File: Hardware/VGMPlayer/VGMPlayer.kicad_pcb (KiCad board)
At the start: 2 copper layers, 110.7 x 70.6 mm, 92 parts, among them J1 USB_B_Mini, J2 SD_Card, Q1 9013, Q2 S8550, SW1 Mode, SW2 NEXT, SW3 PREV, SW4 SELECT, SW5 PWR, U1 STM32F103XX, U10 LTC6903, U11 HC-06, U13 YM3012, U14 LM324, U18 OLED_128_64_I2C, U19 ESP8266Module, U2 SDCardModule, U3 LM386, U4 LM386, U5 YM2151, U6 AUDIOJACK-VGM, U7 YM2612, U8 SN76489, U9 LTC6903

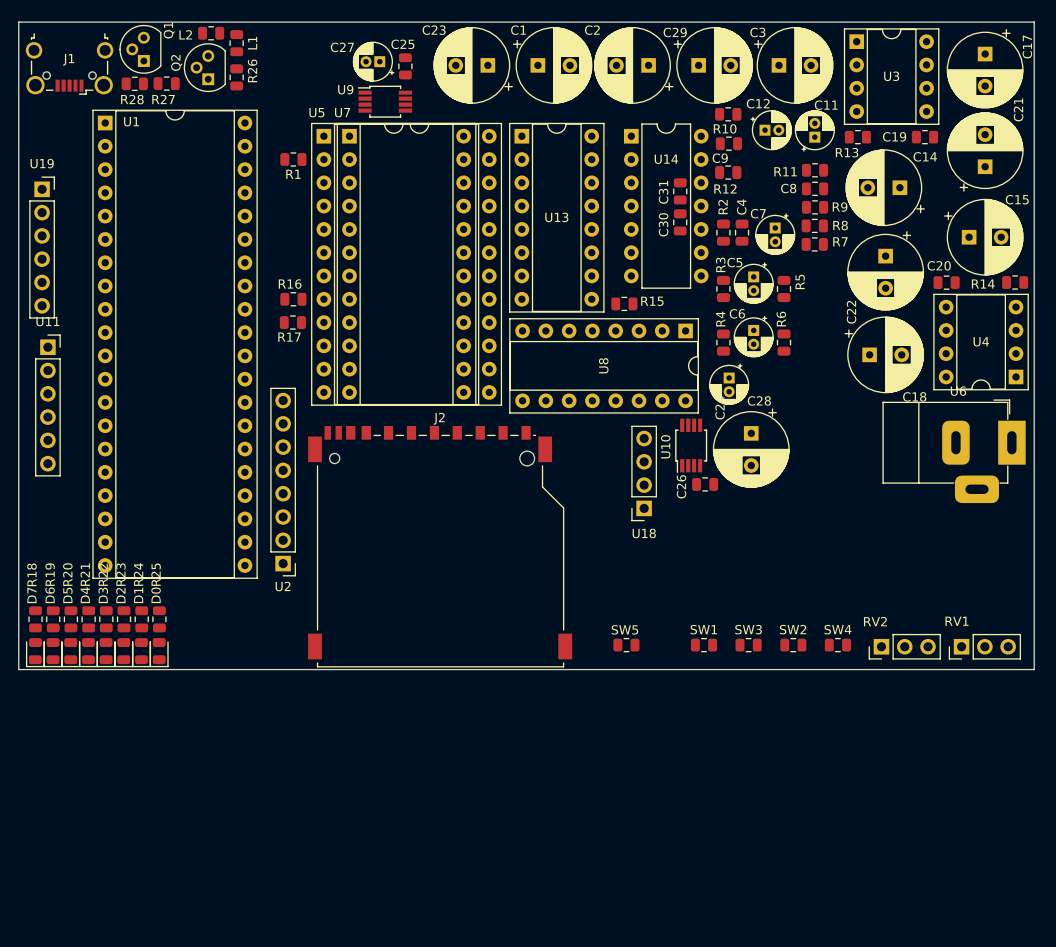
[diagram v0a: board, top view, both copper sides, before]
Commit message: 1
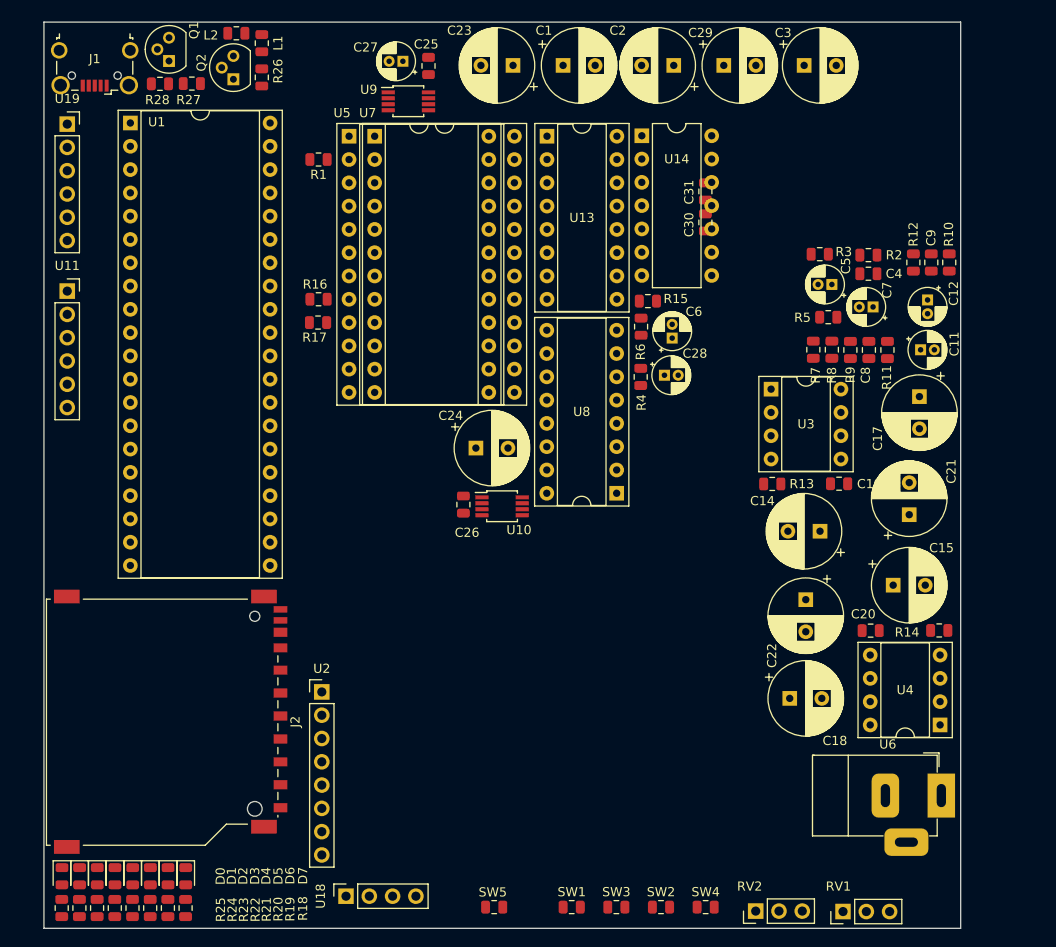
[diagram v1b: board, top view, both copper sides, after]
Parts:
- moved U18 53.3 mm to (53.0, 117.7), turned to 90 degrees
- moved U6 39.2 mm to (117.9, 106.7)
- moved U3 39.0 mm to (99.3, 62.4)
- moved R13 39.0 mm to (99.4, 72.7)
- moved C19 38.9 mm to (106.7, 72.7)
- moved U4 38.8 mm to (117.7, 99.0)
- moved C20 38.8 mm to (110.2, 88.7)
- moved C21 38.8 mm to (114.4, 76.1)
- moved C15 38.8 mm to (112.6, 83.8)
- moved R14 38.8 mm to (117.7, 88.7)
- moved C18 38.5 mm to (101.3, 96.1)
- moved C22 38.5 mm to (103.1, 85.3)
- moved C14 38.5 mm to (104.7, 77.9)
- moved C17 38.0 mm to (115.5, 63.2)
- moved R18 35.5 mm to (35.5, 119.0), turned to 270 degrees
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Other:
- board size 110.7 x 70.6 mm -> 100 x 98.8 mm

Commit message: 1
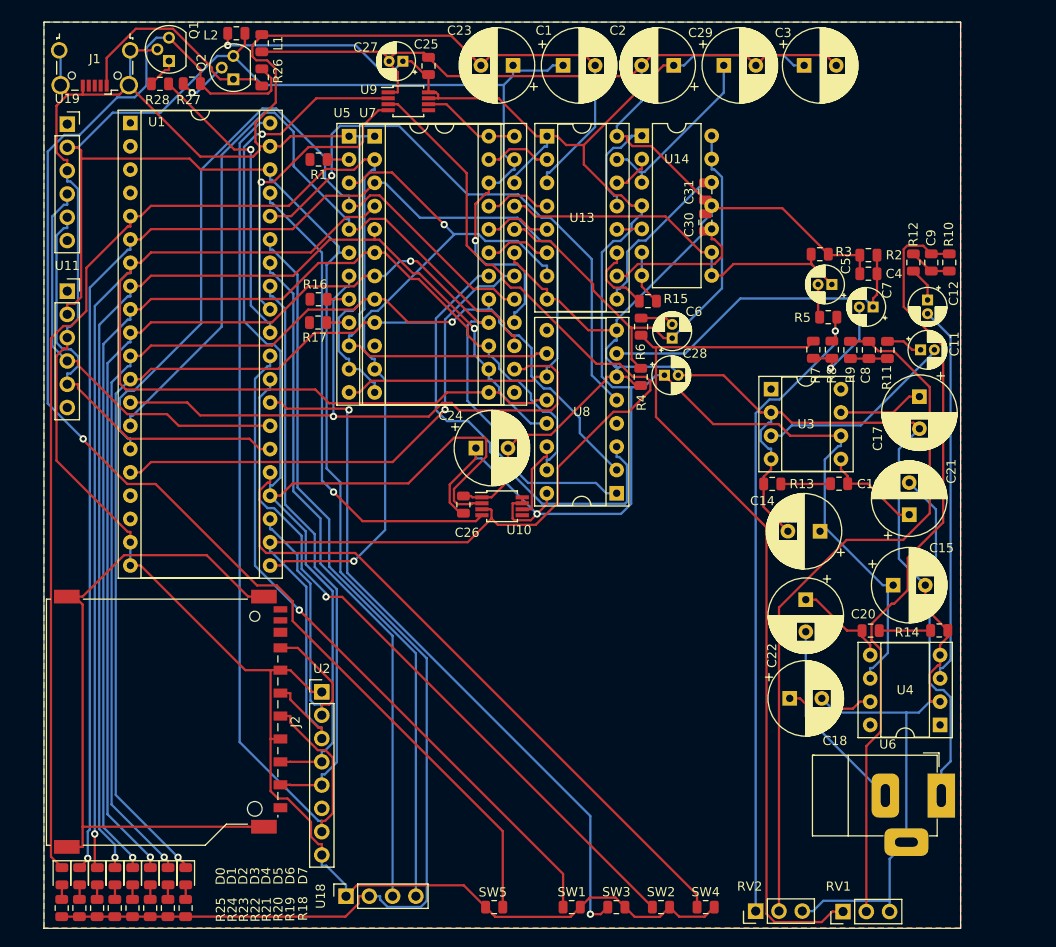
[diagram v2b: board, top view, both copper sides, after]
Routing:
- net GNDA: track 0.00 -> 316.8 mm
- net GND: track 0.00 -> 312.6 mm
- net VDD: track 0.00 -> 272.0 mm, vias 0 -> 1
- net +5V: track 0.00 -> 229.0 mm, vias 0 -> 2
- net D1: track 0.00 -> 160.0 mm, vias 0 -> 1
- net D2: track 0.00 -> 159.4 mm, vias 0 -> 1
- net D0: track 0.00 -> 149.0 mm
- net Net-(Q1-Pad3): track 0.00 -> 144.3 mm, vias 0 -> 1
- net D7: track 0.00 -> 143.0 mm, vias 0 -> 1
- net D5: track 0.00 -> 139.1 mm, vias 0 -> 2
- net SPI_MOSI: track 0.00 -> 133.4 mm, vias 0 -> 1
- net SPI_CLK: track 0.00 -> 131.9 mm
- net D4: track 0.00 -> 128.2 mm, vias 0 -> 1
- net D6: track 0.00 -> 128.0 mm, vias 0 -> 2
- net D3: track 0.00 -> 125.3 mm, vias 0 -> 2
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- added copper zone on B.Cu, net (none)
- added copper zone on F.Cu, net (none)
- added copper zone on F.Cu, net GND
